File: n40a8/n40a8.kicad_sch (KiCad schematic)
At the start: 93 parts, among them J1 Conn_01x16, SW1 SW_Push, SW10 SW_Push, SW11 SW_Push, SW12 SW_Push, SW13 SW_Push, SW14 SW_Push, SW15 SW_Push, SW16 SW_Push, SW17 SW_Push, SW18 SW_Push, SW19 SW_Push, SW2 SW_Push, SW20 SW_Push, SW21 SW_Push, SW22 SW_Push, SW23 SW_Push, SW24 SW_Push, SW25 SW_Push, SW26 SW_Push, SW27 SW_Push, SW28 SW_Push, SW29 SW_Push, SW3 SW_Push, SW30 SW_Push, SW31 SW_Push, SW32 SW_Push, SW33 SW_Push, SW34 SW_Push, SW35 SW_Push, SW36 SW_Push, SW37 SW_Push, SW38 SW_Push, SW39 SW_Push, SW4 SW_Push, SW40 SW_Push, SW41 SW_Push, SW42 SW_Push, SW43 SW_RST, SW44 SW_PWR, SW5 SW_Push, SW6 SW_Push, SW7 SW_Push, SW8 SW_Push, SW9 SW_Push, U1 BLE-Micro-Pro-2, U2 TPS61221

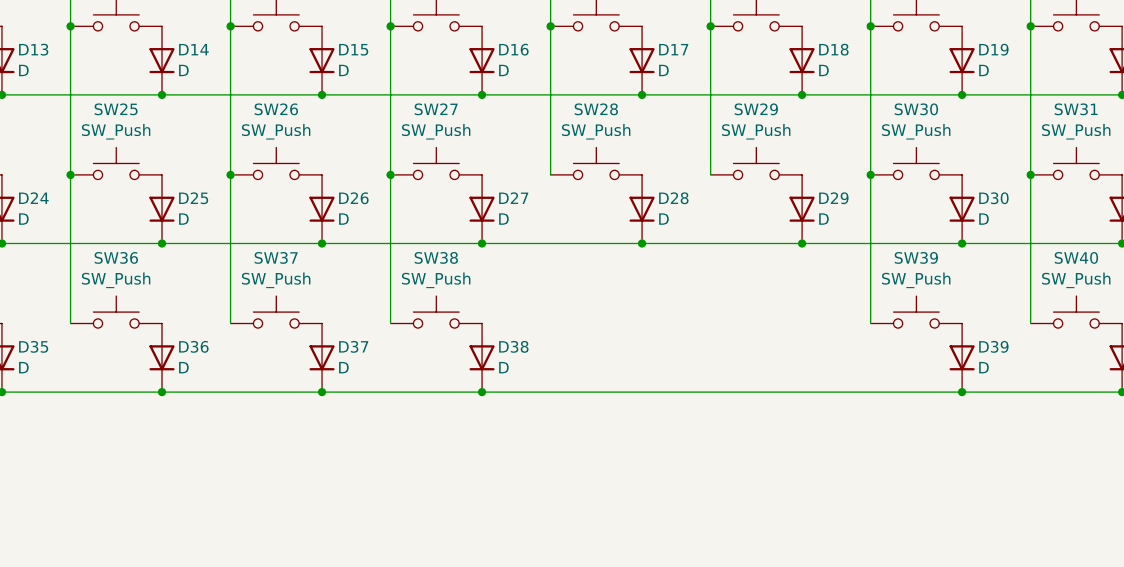
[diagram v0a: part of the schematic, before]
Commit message: wired
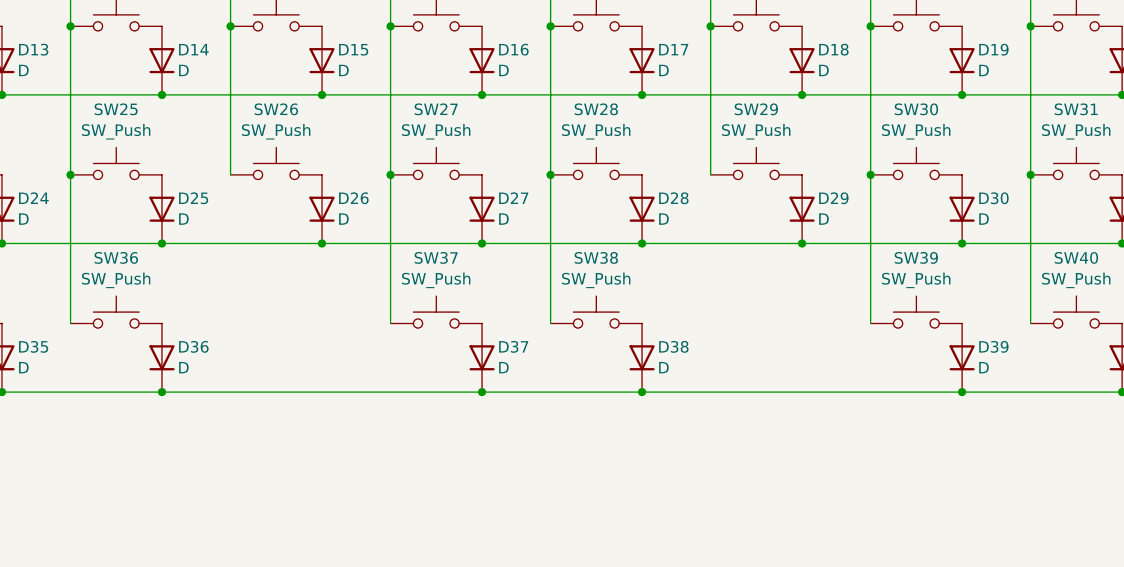
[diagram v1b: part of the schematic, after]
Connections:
- net C2: no longer SW37.1
- net C3: now also SW37.1; no longer SW38.1
- net C4: now also SW38.1
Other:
- moved on the sheet: D37, D38, SW37, SW38
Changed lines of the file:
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@@
 	)
 	(junction
-		(at 71.12 128.27)
-		(diameter 0)
-		(color 0 0 0 0)
-	)
-	(junction
 		(at 185.42 87.63)
 		(diameter 0)
@@
 	)
 	(junction
-		(at 78.74 104.14)
+		(at 96.52 71.12)
 		(diameter 0)
 		(color 0 0 0 0)
 	)
 	(junction
-		(at 96.52 71.12)
+		(at 106.68 128.27)
 		(diameter 0)
 		(color 0 0 0 0)
@@
 	)
 	(junction
+		(at 88.9 128.27)
+		(diameter 0)
+		(color 0 0 0 0)
+	)
+	(junction
 		(at 167.64 71.12)
 		(diameter 0)
@@
 	)
 	(junction
+		(at 78.74 104.14)
+		(diameter 0)
+		(color 0 0 0 0)
+	)
+	(junction
 		(at 29.21 176.53)
 		(diameter 0)
@@
 	)
 	(junction
-		(at 88.9 128.27)
-		(diameter 0)
-		(color 0 0 0 0)
-	)
-	(junction
 		(at 35.56 78.74)
 		(diameter 0)
@@
 	)
 	(junction
-		(at 60.96 104.14)
+		(at 160.02 95.25)
 		(diameter 0)
 		(color 0 0 0 0)
 	)
 	(junction
-		(at 160.02 95.25)
+		(at 96.52 104.14)
 		(diameter 0)
 		(color 0 0 0 0)
@@
 	(wire
 		(pts
-			(xy 203.2 71.12) (xy 203.2 87.63)
+			(xy 106.68 128.27) (xy 142.24 128.27)
 		)
 		(stroke
@@
 	(wire
 		(pts
-			(xy 60.96 48.26) (xy 66.04 48.26)
+			(xy 203.2 71.12) (xy 203.2 87.63)
 		)
 		(stroke
@@
 	(wire
 		(pts
-			(xy 177.8 111.76) (xy 195.58 111.76)
+			(xy 60.96 48.26) (xy 66.04 48.26)
 		)
 		(stroke
@@
 	(wire
 		(pts
-			(xy 40.64 167.64) (xy 62.23 167.64)
+			(xy 177.8 111.76) (xy 195.58 111.76)
 		)
 		(stroke
@@
 	(wire
 		(pts
-			(xy 269.24 55.88) (xy 269.24 54.61)
+			(xy 40.64 167.64) (xy 62.23 167.64)
 		)
 		(stroke
@@
 	(wire
 		(pts
-			(xy 106.68 78.74) (xy 124.46 78.74)
+			(xy 269.24 55.88) (xy 269.24 54.61)
 		)
 		(stroke
@@
 	(wire
 		(pts
-			(xy 63.5 181.61) (xy 63.5 182.88)
+			(xy 106.68 78.74) (xy 124.46 78.74)
 		)
 		(stroke
@@
 	(wire
 		(pts
-			(xy 231.14 78.74) (xy 241.3 78.74)
+			(xy 63.5 181.61) (xy 63.5 182.88)
 		)
 		(stroke
@@
 	(wire
 		(pts
-			(xy 60.96 104.14) (xy 60.96 120.65)
+			(xy 231.14 78.74) (xy 241.3 78.74)
 		)
 		(stroke
@@
 	(wire
 		(pts
-			(xy 53.34 128.27) (xy 71.12 128.27)
+			(xy 53.34 128.27) (xy 88.9 128.27)
 		)
 		(stroke
@@
 	(wire
 		(pts
-			(xy 149.86 71.12) (xy 149.86 87.63)
+			(xy 78.74 104.14) (xy 78.74 120.65)
 		)
 		(stroke
@@
 	(wire
 		(pts
-			(xy 88.9 95.25) (xy 106.68 95.25)
+			(xy 149.86 71.12) (xy 149.86 87.63)
 		)
 		(stroke
@@
 	(wire
 		(pts
-			(xy 71.12 128.27) (xy 88.9 128.27)
+			(xy 88.9 95.25) (xy 106.68 95.25)
 		)
 		(stroke
@@
 	(wire
 		(pts
+			(xy 88.9 128.27) (xy 106.68 128.27)
+		)
+		(stroke
+			(width 0)
+			(type default)
+		)
+	)
+	(wire
+		(pts
 			(xy 177.8 78.74) (xy 195.58 78.74)
 		)
@@
 	(wire
 		(pts
-			(xy 88.9 128.27) (xy 142.24 128.27)
-		)
-		(stroke
-			(width 0)
-			(type default)
-		)
-	)
-	(wire
-		(pts
 			(xy 38.1 189.23) (xy 38.1 190.5)
 		)
@@
 	(wire
 		(pts
+			(xy 96.52 104.14) (xy 96.52 120.65)
+		)
+		(stroke
+			(width 0)
+			(type default)
+		)
+	)
+	(wire
+		(pts
 			(xy 60.96 50.8) (xy 66.04 50.8)
 		)
@@
 	(wire
 		(pts
-			(xy 78.74 104.14) (xy 78.74 120.65)
-		)
-		(stroke
-			(width 0)
-			(type default)
-		)
-	)
-	(wire
-		(pts
 			(xy 78.74 63.5) (xy 78.74 71.12)
 		)
@@
 	(symbol
 		(lib_id "Switch:SW_Push")
-		(at 83.82 120.65 0)
+		(at 101.6 120.65 0)
 		(unit 1)
 		(exclude_from_sim no)
@@
 		(dnp no)
 		(property "Reference" "SW38"
-			(at 83.82 113.411 0)
+			(at 101.6 113.411 0)
 			(effects
 				(font
@@
 		)
 		(property "Value" "SW_Push"
-			(at 83.82 115.7224 0)
+			(at 101.6 115.7224 0)
 			(effects
 				(font
@@
 		)
 		(property "Footprint" "cscslib:CPG151101S11_2u"
-			(at 83.82 115.57 0)
+			(at 101.6 115.57 0)
 			(effects
 				(font
@@
 		)
 		(property "Datasheet" ""
-			(at 83.82 115.57 0)
+			(at 101.6 115.57 0)
 			(effects
 				(font
@@
 		)
 		(property "Description" ""
-			(at 83.82 120.65 0)
+			(at 101.6 120.65 0)
 			(effects
 				(font
@@
 	(symbol
 		(lib_id "Switch:SW_Push")
-		(at 66.04 120.65 0)
+		(at 83.82 120.65 0)
 		(unit 1)
 		(exclude_from_sim no)
@@
 		(dnp no)
 		(property "Reference" "SW37"
-			(at 66.04 113.411 0)
+			(at 83.82 113.411 0)
 			(effects
 				(font
@@
 		)
 		(property "Value" "SW_Push"
-			(at 66.04 115.7224 0)
+			(at 83.82 115.7224 0)
 			(effects
 				(font
@@
 		)
 		(property "Footprint" "cscslib:CPG151101S11_1.25u"
-			(at 66.04 115.57 0)
+			(at 83.82 115.57 0)
 			(effects
 				(font
@@
 		)
 		(property "Datasheet" ""
-			(at 66.04 115.57 0)
+			(at 83.82 115.57 0)
 			(effects
 				(font
@@
 		)
 		(property "Description" ""
-			(at 66.04 120.65 0)
+			(at 83.82 120.65 0)
 			(effects
 				(font
@@
 	(symbol
 		(lib_id "Diode:1N4148W")
-		(at 88.9 124.46 90)
+		(at 106.68 124.46 90)
 		(unit 1)
 		(exclude_from_sim no)
@@
 		(dnp no)
 		(property "Reference" "D38"
-			(at 90.6272 123.2916 90)
+			(at 108.4072 123.2916 90)
 			(effects
 				(font
@@
 		)
 		(property "Value" "D"
-			(at 90.6272 125.603 90)
+			(at 108.4072 125.603 90)
 			(effects
 				(font
@@
 		)
 		(property "Footprint" "Diode_SMD:D_SOD-123"
-			(at 93.345 124.46 0)
+			(at 111.125 124.46 0)
 			(effects
 				(font
@@
 		)
 		(property "Datasheet" "https://www.vishay.com/docs/85748/1n4148w.pdf"
-			(at 88.9 124.46 0)
+			(at 106.68 124.46 0)
 			(effects
 				(font
@@
 		)
 		(property "Description" "75V 0.15A Fast Switching Diode, SOD-123"
-			(at 88.9 124.46 0)
+			(at 106.68 124.46 0)
 			(effects
 				(font
@@
 		)
 		(property "Sim.Device" "D"
-			(at 88.9 124.46 0)
+			(at 106.68 124.46 0)
 			(effects
 				(font
@@
 		)
 		(property "Sim.Pins" "1=K 2=A"
-			(at 88.9 124.46 0)
+			(at 106.68 124.46 0)
 			(effects
 				(font
@@
 	(symbol
 		(lib_id "Diode:1N4148W")
-		(at 71.12 124.46 90)
+		(at 88.9 124.46 90)
 		(unit 1)
 		(exclude_from_sim no)
@@
 		(dnp no)
 		(property "Reference" "D37"
-			(at 72.8472 123.2916 90)
+			(at 90.6272 123.2916 90)
 			(effects
 				(font
@@
 		)
 		(property "Value" "D"
-			(at 72.8472 125.603 90)
+			(at 90.6272 125.603 90)
 			(effects
 				(font
@@
 		)
 		(property "Footprint" "Diode_SMD:D_SOD-123"
-			(at 75.565 124.46 0)
+			(at 93.345 124.46 0)
 			(effects
 				(font
@@
 		)
 		(property "Datasheet" "https://www.vishay.com/docs/85748/1n4148w.pdf"
-			(at 71.12 124.46 0)
+			(at 88.9 124.46 0)
 			(effects
 				(font
@@
 		)
 		(property "Description" "75V 0.15A Fast Switching Diode, SOD-123"
-			(at 71.12 124.46 0)
+			(at 88.9 124.46 0)
 			(effects
 				(font
@@
 		)
 		(property "Sim.Device" "D"
-			(at 71.12 124.46 0)
+			(at 88.9 124.46 0)
 			(effects
 				(font
@@
 		)
 		(property "Sim.Pins" "1=K 2=A"
-			(at 71.12 124.46 0)
+			(at 88.9 124.46 0)
 			(effects
 				(font

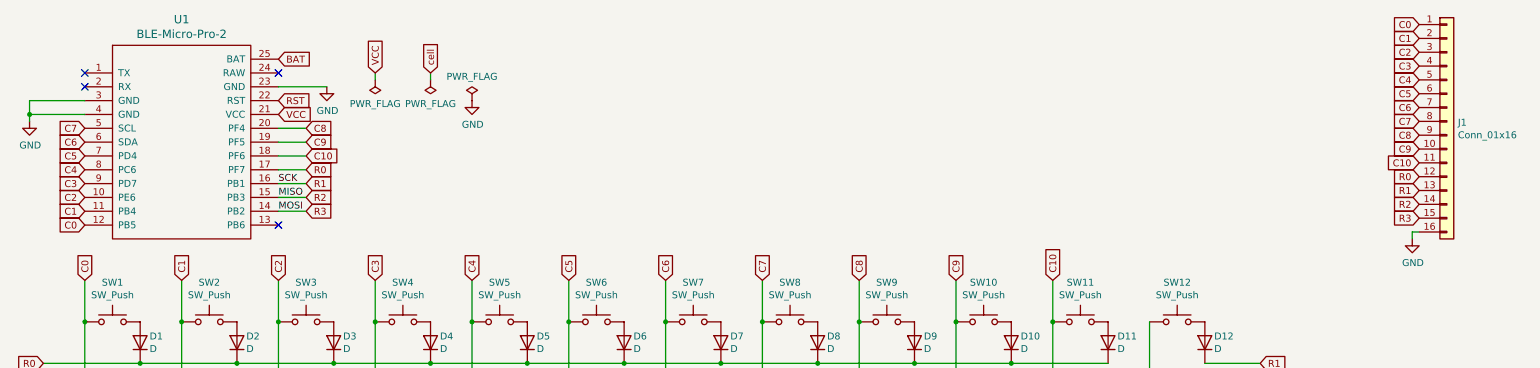
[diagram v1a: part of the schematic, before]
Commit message: wiring complete
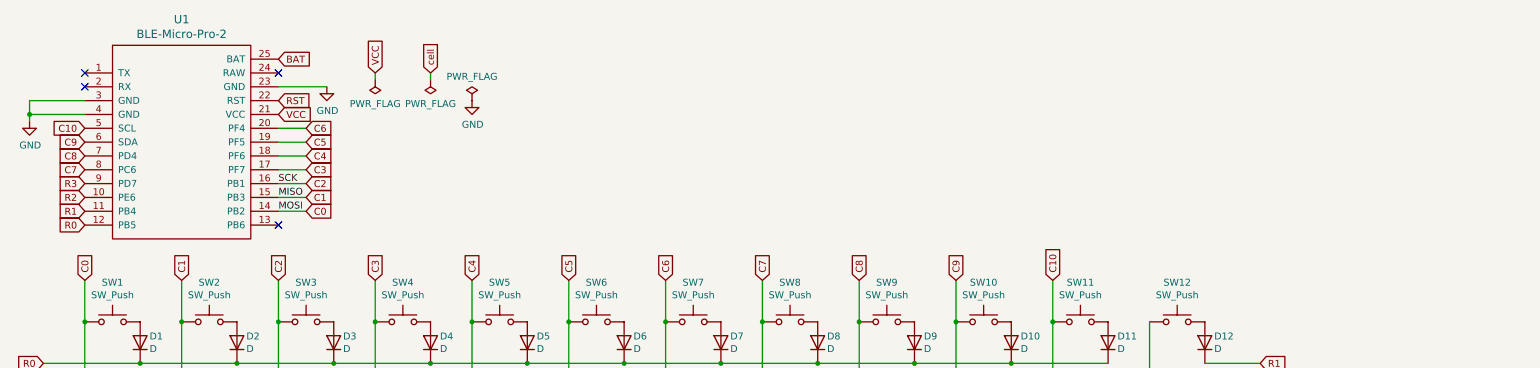
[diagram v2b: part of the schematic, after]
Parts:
- removed J1: Conn_01x16, cscslib:PinHeader_1x16_P1.27mm_Conthrough, symbol Connector_Generic:Conn_01x16
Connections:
- net C0: now also U1.14 (PB2); no longer U1.12 (PB5)
- net C1: now also U1.15 (PB3); no longer U1.11 (PB4)
- net C10: now also U1.5 (SCL); no longer U1.18 (PF6)
- net C2: now also U1.16 (PB1); no longer U1.10 (PE6)
- net C3: now also U1.17 (PF7); no longer U1.9 (PD7)
- net C4: now also U1.18 (PF6); no longer U1.8 (PC6)
- net C5: now also U1.19 (PF5); no longer U1.7 (PD4)
- net C6: now also U1.20 (PF4); no longer U1.6 (SDA)
- net C7: now also U1.8 (PC6); no longer U1.5 (SCL)
- net C8: now also U1.7 (PD4); no longer U1.20 (PF4)
- net C9: now also U1.6 (SDA); no longer U1.19 (PF5)
- net R0: now also U1.12 (PB5); no longer U1.17 (PF7)
- net R1: now also U1.11 (PB4); no longer U1.16 (PB1)
- net R2: now also U1.10 (PE6); no longer U1.15 (PB3)
- net R3: now also U1.9 (PD7); no longer U1.14 (PB2)
